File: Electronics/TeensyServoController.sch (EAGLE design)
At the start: 17 parts, among them U1 MK20DX128VLH5, U2 AP3211_SWITCHING_REGULATOR, U3 AP3211_SWITCHING_REGULATOR, U4 AP3211_SWITCHING_REGULATOR

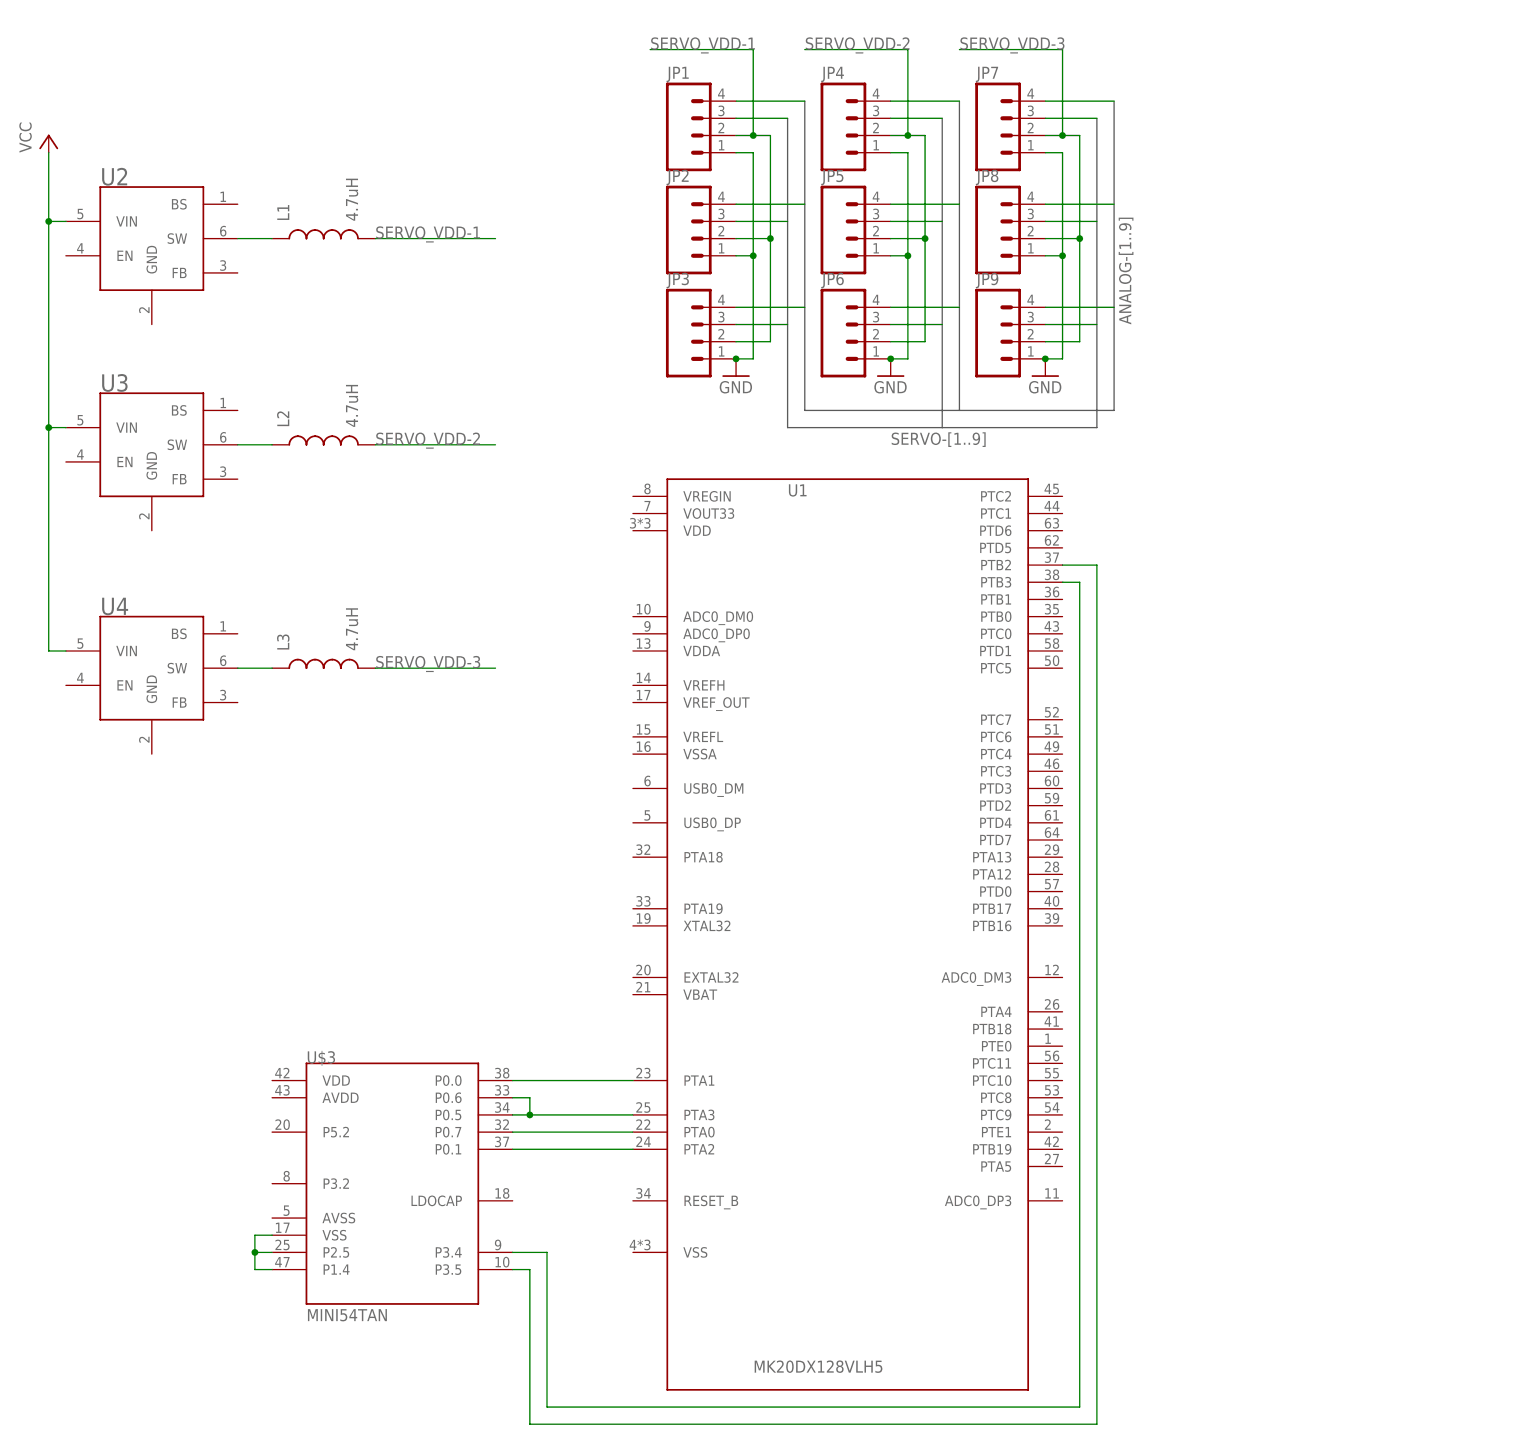
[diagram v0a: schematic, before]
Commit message: Continued Work on Teensy servo controller
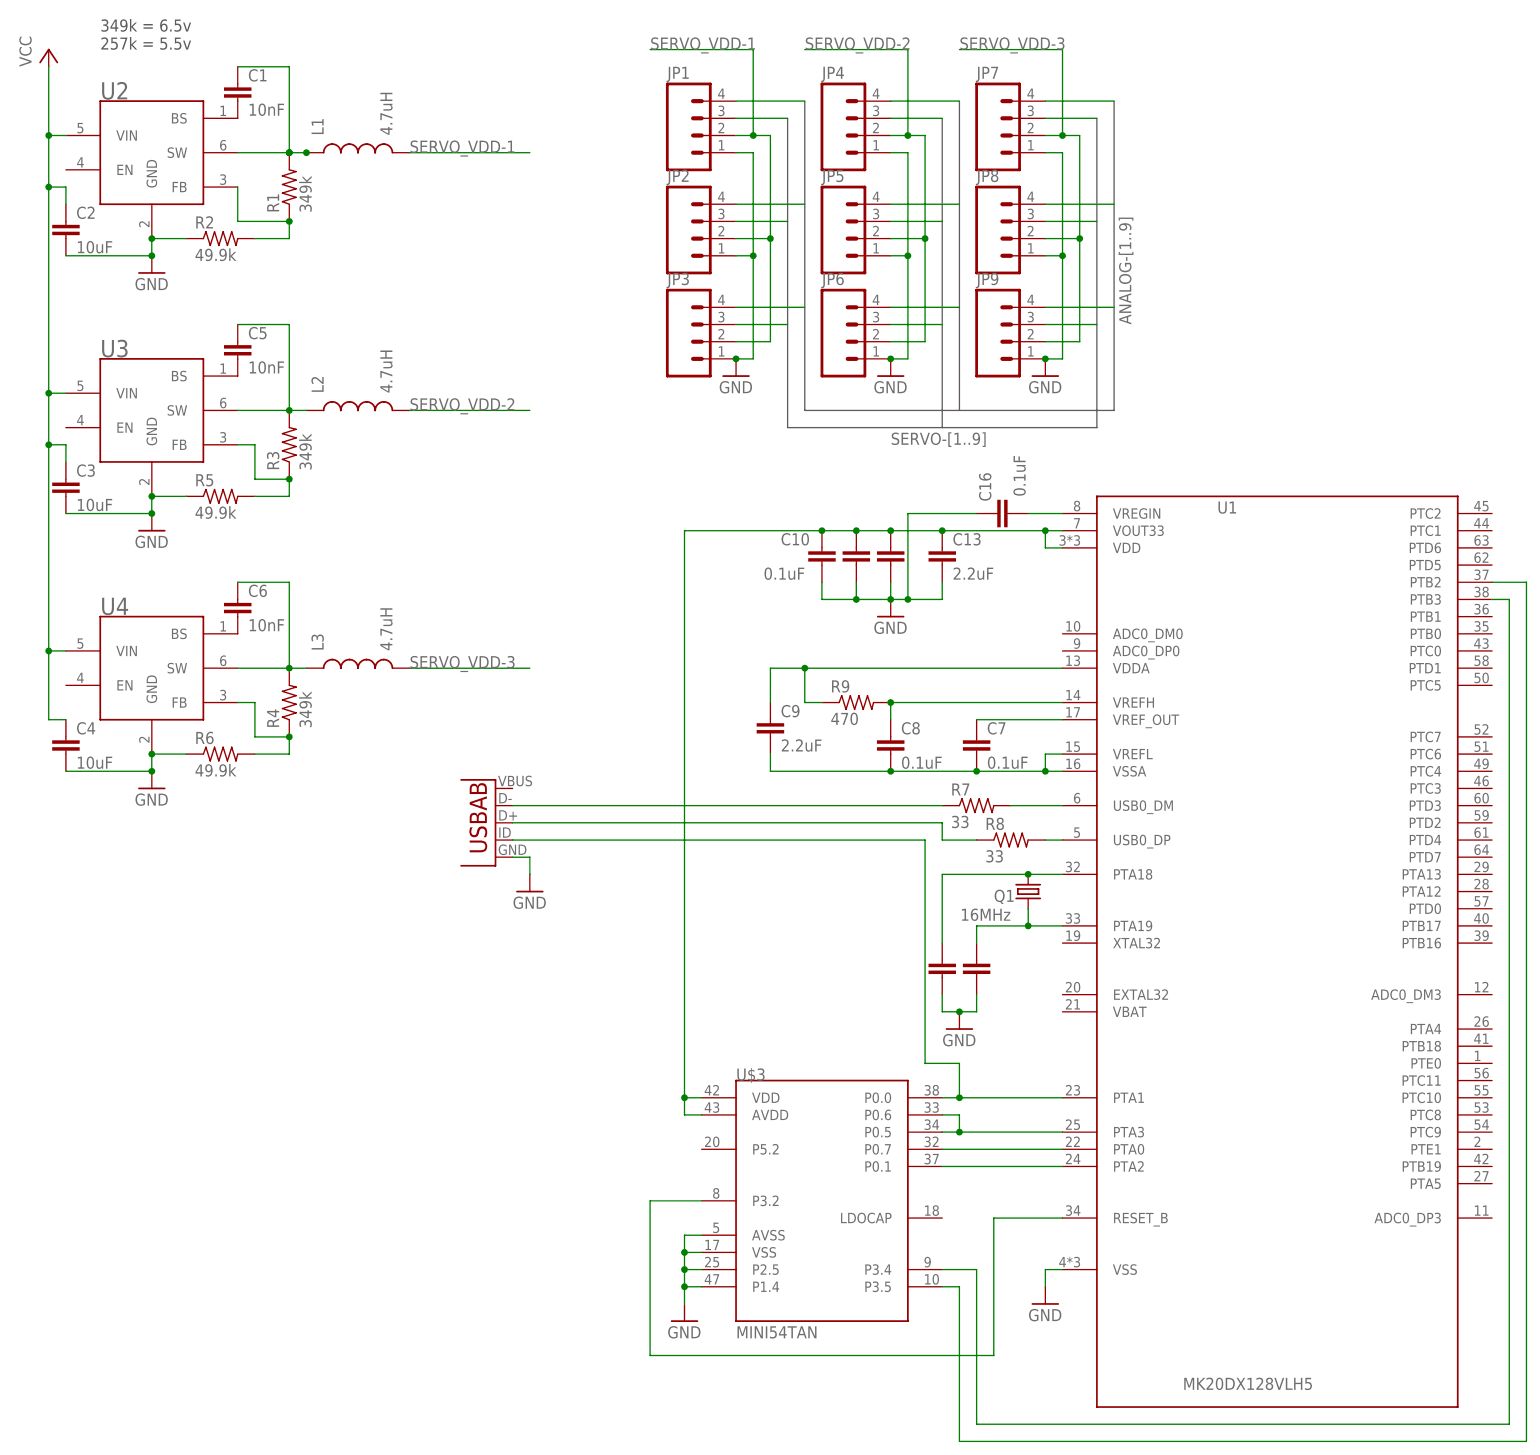
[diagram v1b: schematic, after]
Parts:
- added C1, C5, C6: 10nF, resistor:C-EUC0402
- added C10, C11, C12, C14, C15, C16, C7, C8: 0.1uF, resistor:C-EUC0402
- added C13, C9: 2.2uF, resistor:C-EUC0603
- added C2, C3, C4: 10uF, resistor:C-EUC0805
- added Q1: 16MHz, crystal:CRYSTALCTS406
- added R1, R3, R4: 349k, resistor:R-US_R0402
- added R2, R5, R6: 49.9k, resistor:R-US_R0402
- added R7, R8: 33, resistor:R-US_R0402
- added R9: 470, resistor:R-US_R0402
- added U5: (no value), SparkFun-Connectors:USB-AB
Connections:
- removed net N$8: U$3.P1.4, U$3.P2.5, U$3.VSS
- new net N$10: R7.1, U5.D-
- new net N$14: C1.2, U2.BS
- new net N$15: R8.2, U1.USB0_DP
- new net N$16: R4.1, R6.2, U4.FB
- new net N$17: C5.2, U3.BS
- new net N$18: R3.1, R5.2, U3.FB
- new net N$19: C6.2, U4.BS
- new net N$20: C6.1, L3.1, R4.2, U4.SW
- new net N$21: C14.1, Q1.2, U1.PTA18
- new net N$22: C15.1, Q1.1, U1.PTA19
- new net N$23: C16.2, U1.VREGIN
- new net N$24: C9.1, R9.1, U1.VDDA
- new net N$25: C7.2, C8.2, C9.2, U1.VREFL, U1.VSSA
- new net N$26: C7.1, U1.VREF_OUT
- new net N$27: C8.1, R9.2, U1.VREFH
- new net N$30: U$3.P3.2, U1.RESET_B
- new net N$31: C10.1, C11.1, C12.1, C13.1, U$3.AVDD, U$3.VDD, U1.VDD, U1.VOUT33
- new net N$6: R1.1, R2.2, U2.FB
- new net N$9: R8.1, U5.D+
- net GND: now also C10.2, C11.2, C12.2, C13.2, C14.2, C15.2, C16.1, C2.2, C3.2, C4.2, R2.1, R5.1, R6.1, U$3.AVSS, U$3.P1.4, U$3.P2.5, U$3.VSS, U1.VSS, U2.GND, U3.GND, U4.GND, U5.GND
- net N$1: now also U5.USBID
- net N$11: now also C5.1, R3.2
- net N$12: now also R7.2, U1.USB0_DM; no longer L3.1, U4.SW
- net N$13: now also C1.1, R1.2
- net VCC: now also C2.1, C3.1, C4.1
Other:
- note added: "349k = 6.5v 257k = 5.5v"
- moved on the sheet: L1, L2, L3, U$3, U1, U2, U3
